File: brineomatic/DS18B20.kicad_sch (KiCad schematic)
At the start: 5 parts

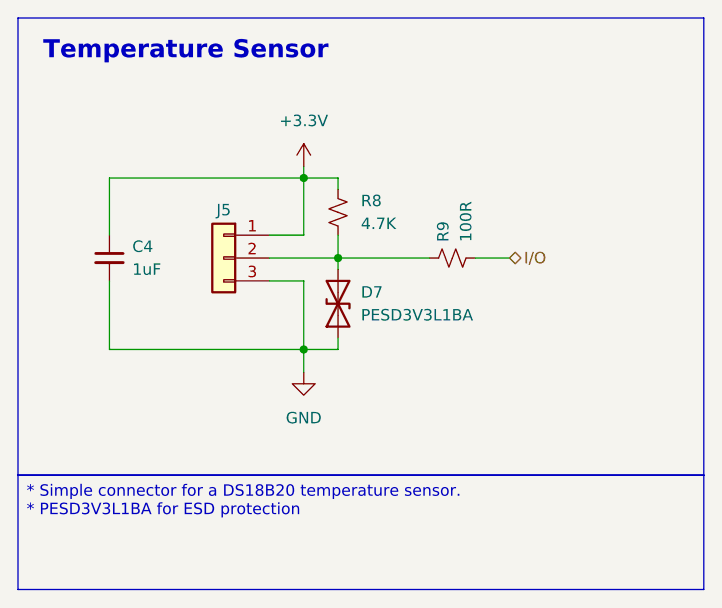
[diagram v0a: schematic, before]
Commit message: added test points
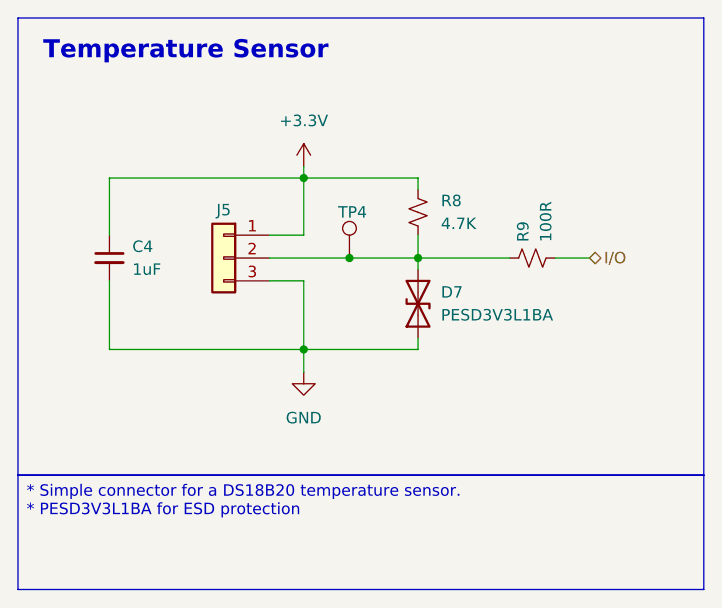
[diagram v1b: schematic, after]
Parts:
- added TP4: TestPoint, TestPoint:TestPoint_Pad_D1.5mm, symbol Connector:TestPoint
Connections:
- net at D7.2 (A2), J5.2 (Pin_2), R8.1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: now also TP4.1
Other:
- moved on the sheet: D7, R8, R9
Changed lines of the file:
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@@
+	)
+	(junction
+		(at 124.46 93.98)
+		(diameter 0)
+		(color 0 0 0 0)
 	)
 	(junction
@@
 	)
 	(junction
-		(at 123.19 93.98)
+		(at 132.08 93.98)
 		(diameter 0)
 		(color 0 0 0 0)
@@
 	(wire
 		(pts
-			(xy 123.19 93.98) (xy 133.35 93.98)
+			(xy 132.08 93.98) (xy 142.24 93.98)
 		)
 		(stroke
@@
 	(wire
 		(pts
-			(xy 123.19 85.09) (xy 123.19 86.36)
+			(xy 132.08 85.09) (xy 132.08 86.36)
 		)
 		(stroke
@@
 	(wire
 		(pts
-			(xy 119.38 104.14) (xy 123.19 104.14)
-		)
-		(stroke
-			(width 0)
-			(type default)
-		)
-	)
-	(wire
-		(pts
-			(xy 119.38 85.09) (xy 123.19 85.09)
-		)
-		(stroke
-			(width 0)
-			(type default)
-		)
-	)
-	(wire
-		(pts
-			(xy 115.57 93.98) (xy 123.19 93.98)
+			(xy 119.38 104.14) (xy 132.08 104.14)
+		)
+		(stroke
+			(width 0)
+			(type default)
+		)
+	)
+	(wire
+		(pts
+			(xy 119.38 85.09) (xy 132.08 85.09)
+		)
+		(stroke
+			(width 0)
+			(type default)
+		)
+	)
+	(wire
+		(pts
+			(xy 115.57 93.98) (xy 124.46 93.98)
 		)
 		(stroke
@@
 	(wire
 		(pts
-			(xy 123.19 91.44) (xy 123.19 93.98)
+			(xy 132.08 91.44) (xy 132.08 93.98)
 		)
 		(stroke
@@
 	(wire
 		(pts
-			(xy 138.43 93.98) (xy 142.24 93.98)
-		)
-		(stroke
-			(width 0)
-			(type default)
-		)
-	)
-	(wire
-		(pts
-			(xy 123.19 95.25) (xy 123.19 93.98)
+			(xy 124.46 93.98) (xy 132.08 93.98)
+		)
+		(stroke
+			(width 0)
+			(type default)
+		)
+	)
+	(wire
+		(pts
+			(xy 147.32 93.98) (xy 151.13 93.98)
+		)
+		(stroke
+			(width 0)
+			(type default)
+		)
+	)
+	(wire
+		(pts
+			(xy 132.08 95.25) (xy 132.08 93.98)
 		)
 		(stroke
@@
 	(wire
 		(pts
-			(xy 123.19 104.14) (xy 123.19 102.87)
+			(xy 132.08 104.14) (xy 132.08 102.87)
 		)
 		(stroke
@@
 	(hierarchical_label "I{slash}O"
 		(shape bidirectional)
-		(at 142.24 93.98 0)
+		(at 151.13 93.98 0)
 		(effects
 			(font
@@
 	(symbol
 		(lib_id "Device:D_TVS")
-		(at 123.19 99.06 90)
+		(at 132.08 99.06 90)
 		(unit 1)
 		(exclude_from_sim no)
@@
 		(dnp no)
 		(property "Reference" "D7"
-			(at 125.73 97.7899 90)
+			(at 134.62 97.7899 90)
 			(effects
 				(font
@@
 		)
 		(property "Value" "PESD3V3L1BA"
-			(at 125.73 100.3299 90)
+			(at 134.62 100.3299 90)
 			(effects
 				(font
@@
 		)
 		(property "Footprint" "Diode_SMD:D_SOD-323"
-			(at 123.19 99.06 0)
+			(at 132.08 99.06 0)
 			(effects
 				(font
@@
 		)
 		(property "Datasheet" "~"
-			(at 123.19 99.06 0)
+			(at 132.08 99.06 0)
 			(effects
 				(font
@@
 		)
 		(property "Description" "Bidirectional transient-voltage-suppression diode"
-			(at 123.19 99.06 0)
+			(at 132.08 99.06 0)
 			(effects
 				(font
@@
 		)
 		(property "LCSC Part Name" ""
-			(at 123.19 99.06 90)
+			(at 132.08 99.06 90)
 			(effects
 				(font
@@
 		)
 		(property "Manufacturer" ""
-			(at 123.19 99.06 90)
+			(at 132.08 99.06 90)
 			(effects
 				(font
@@
 		)
 		(property "Manufacturer Part" ""
-			(at 123.19 99.06 90)
+			(at 132.08 99.06 90)
 			(effects
 				(font
@@
 		)
 		(property "Supplier" ""
-			(at 123.19 99.06 90)
+			(at 132.08 99.06 90)
 			(effects
 				(font
@@
 		)
 		(property "Supplier Part" ""
-			(at 123.19 99.06 90)
+			(at 132.08 99.06 90)
 			(effects
 				(font
@@
 		)
 		(property "LCSC" "C2687129"
-			(at 123.19 99.06 90)
+			(at 132.08 99.06 90)
 			(effects
 				(font
@@
 	)
 	(symbol
+		(lib_id "Connector:TestPoint")
+		(at 124.46 93.98 0)
+		(unit 1)
+		(exclude_from_sim no)
+		(in_bom yes)
+		(on_board yes)
+		(dnp no)
+		(property "Reference" "TP4"
+			(at 123.19 88.9 0)
+			(effects
+				(font
+					(size 1.27 1.27)
+				)
+				(justify left)
+			)
+		)
+		(property "Value" "TestPoint"
+			(at 127 91.9479 0)
+			(effects
+				(font
+					(size 1.27 1.27)
+				)
+				(justify left)
+				(hide yes)
+			)
+		)
+		(property "Footprint" "TestPoint:TestPoint_Pad_D1.5mm"
+			(at 129.54 93.98 0)
+			(effects
+				(font
+					(size 1.27 1.27)
+				)
+				(hide yes)
+			)
+		)
+		(property "Datasheet" "~"
+			(at 129.54 93.98 0)
+			(effects
+				(font
+					(size 1.27 1.27)
+				)
+				(hide yes)
+			)
+		)
+		(property "Description" "test point"
+			(at 124.46 93.98 0)
+			(effects
+				(font
+					(size 1.27 1.27)
+				)
+				(hide yes)
+			)
+		)
+		(pin "1"
+		)
+		(instances
+			(project "brineomatic"
+				(path "/96477ae2-ef08-48f3-8dd4-fe4478541f68/4c28a3dc-9363-4fde-b010-be952dc8ce44"
+					(reference "TP35")
+					(unit 1)
+				)
+				(path "/96477ae2-ef08-48f3-8dd4-fe4478541f68/7dc38cc9-02c6-4108-8c2f-d0f758210cae"
+					(reference "TP4")
+					(unit 1)
+				)
+			)
+		)
+	)
+	(symbol
 		(lib_id "Device:R_Small_US")
-		(at 135.89 93.98 270)
+		(at 144.78 93.98 270)
 		(unit 1)
 		(exclude_from_sim no)
@@
 		(dnp no)
 		(property "Reference" "R9"
-			(at 134.874 92.202 0)
+			(at 143.764 92.202 0)
 			(effects
 				(font
@@
 		)
 		(property "Value" "100R"
-			(at 137.414 92.202 0)
+			(at 146.304 92.202 0)
 			(effects
 				(font
@@
 		)
 		(property "Footprint" "Resistor_SMD:R_0603_1608Metric"
-			(at 135.89 93.98 0)
+			(at 144.78 93.98 0)
 			(effects
 				(font
@@
 		)
 		(property "Datasheet" "~"
-			(at 135.89 93.98 0)
+			(at 144.78 93.98 0)
 			(effects
 				(font
@@
 		)
 		(property "Description" "Resistor, small US symbol"
-			(at 135.89 93.98 0)
+			(at 144.78 93.98 0)
 			(effects
 				(font
@@
 		)
 		(property "LCSC" ""
-			(at 135.89 93.98 0)
+			(at 144.78 93.98 0)
 			(effects
 				(font
@@
 	(symbol
 		(lib_id "Device:R_Small_US")
-		(at 123.19 88.9 180)
+		(at 132.08 88.9 180)
 		(unit 1)
 		(exclude_from_sim no)
@@
 		(fields_autoplaced yes)
 		(property "Reference" "R8"
-			(at 125.73 87.6299 0)
+			(at 134.62 87.6299 0)
 			(effects
 				(font
@@
 		)
 		(property "Value" "4.7K"
-			(at 125.73 90.1699 0)
+			(at 134.62 90.1699 0)
 			(effects
 				(font
@@
 		)
 		(property "Footprint" "Resistor_SMD:R_0603_1608Metric"
-			(at 123.19 88.9 0)
+			(at 132.08 88.9 0)
 			(effects
 				(font
@@
 		)
 		(property "Datasheet" "~"
-			(at 123.19 88.9 0)
+			(at 132.08 88.9 0)
 			(effects
 				(font
@@
 		)
 		(property "Description" "Resistor, small US symbol"
-			(at 123.19 88.9 0)
+			(at 132.08 88.9 0)
 			(effects
 				(font
@@
 		)
 		(property "LCSC" " C23162"
-			(at 123.19 88.9 0)
-			(effects
-				(font
+			(at 132.08 88.9 0)
+			(effects
+				(font

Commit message: bom and placement verified
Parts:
- C4: LCSC (none) -> C15849
- R9: LCSC (none) -> C22775
- TP4: now left out of the parts list
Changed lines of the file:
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@@
+			)
+		)
+		(property "LCSC" "C15849"
+			(at 97.79 93.98 0)
+			(effects
+				(font
+					(size 1.27 1.27)
+				)
+				(hide yes)
 			)
 		)
@@
 		(unit 1)
 		(exclude_from_sim no)
-		(in_bom yes)
+		(in_bom no)
 		(on_board yes)
 		(dnp no)
@@
 			)
 		)
-		(property "LCSC" ""
+		(property "LCSC" "C22775"
 			(at 144.78 93.98 0)
 			(effects
